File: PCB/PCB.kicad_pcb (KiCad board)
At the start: 6 copper layers, 22 x 80 mm, 269 parts, among them J1 Bus_M.2_Edge_M, J2 Conn_ARM_SWD_TagConnect_TC2030, J4 TYPE-C-31-M-12, J7 HDMI_D_1.4, SW1 SW_Push, U1 XC7A50T-FGG484, U10 FT2232HQ, U11 MT41J128M16JT-125:K, U12 PCA9306DC1, U14 UCL0524P, U15 UCL0524P, U16 UCL0524P, U17 TPS62132, U2 MAX20029ATIA/V+, U3 TPD2EUSB30, U4 TPD2EUSB30, U5 TPS2121RUXR, U6 TPD2EUSB30, U7 MT25QL128ABA1EW7-0SIT, U9 M93C56-WMN6TP, Y2 12MHz, Y3 100MHz

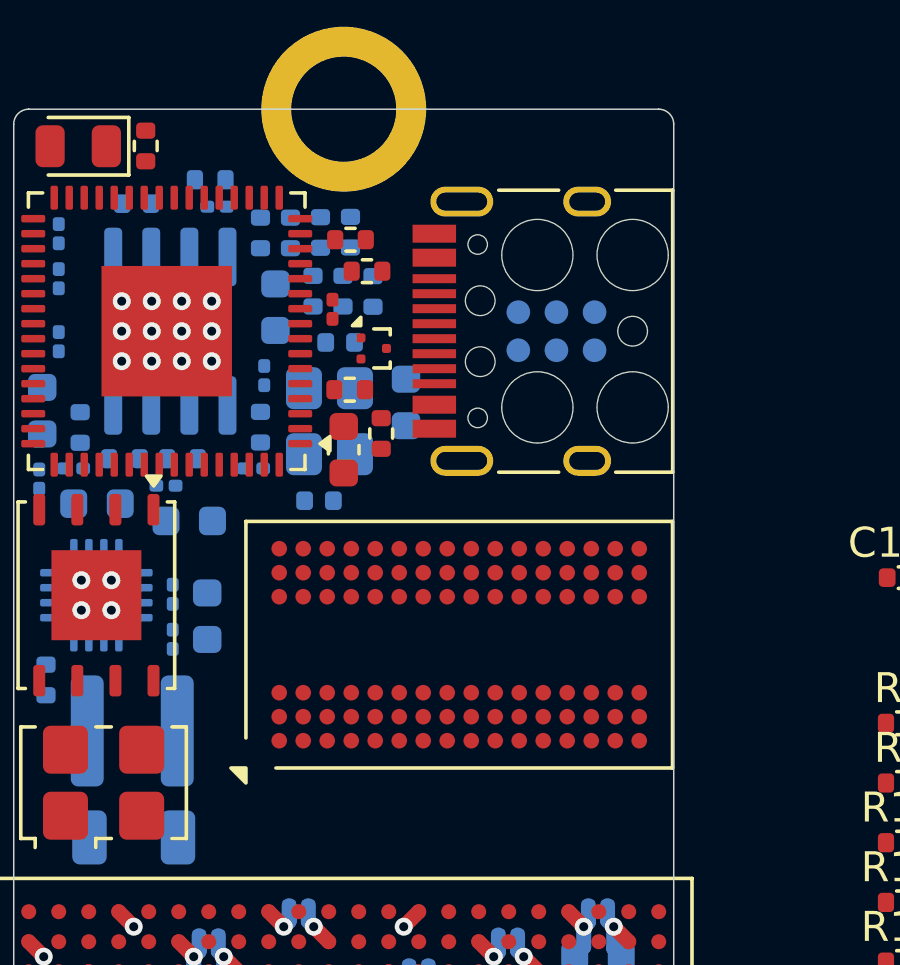
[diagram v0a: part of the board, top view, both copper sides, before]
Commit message: getting ready for DDR routing
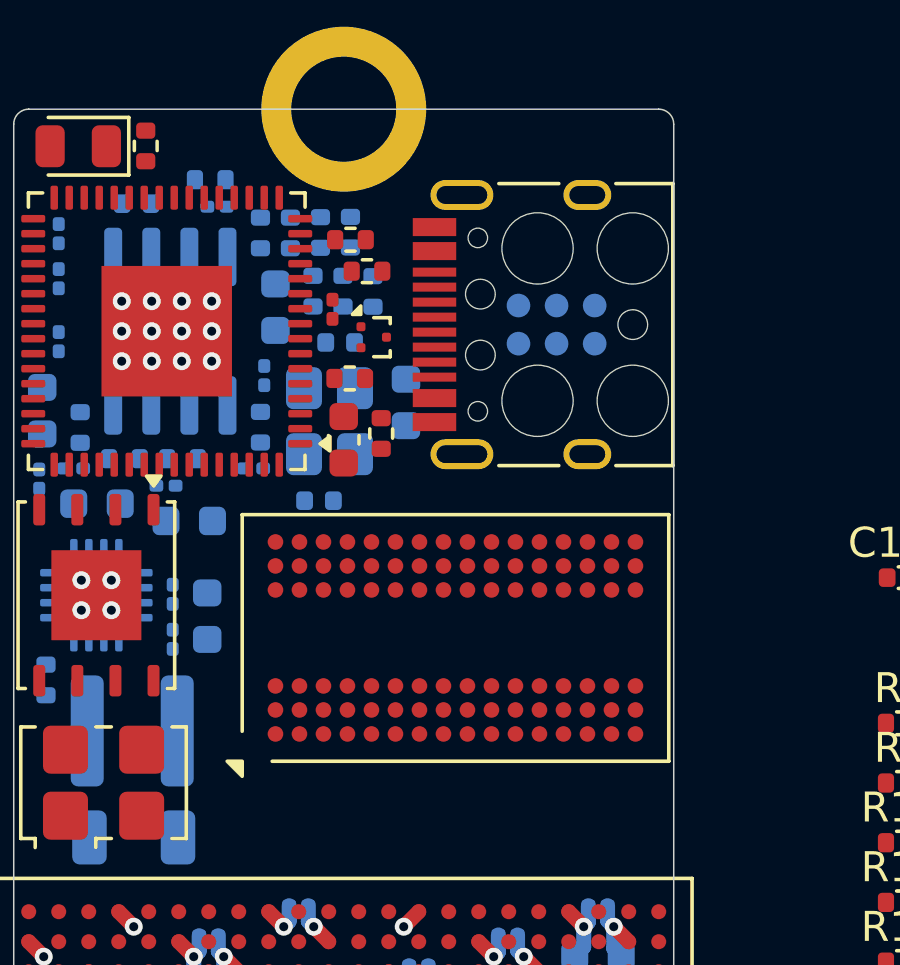
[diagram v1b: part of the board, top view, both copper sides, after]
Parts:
- moved R55 0.38 mm to (143.9, 69.2)
- moved U3 0.38 mm to (144.8, 67.8)
- moved C101 0.33 mm to (143.8, 71.3)
- moved U11 0.26 mm to (147.5, 77.9)
- moved J2 0.22 mm to (150.8, 67.4)
- moved J4 0.22 mm to (150.8, 67.4)
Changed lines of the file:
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@@
 	(footprint "Package_TO_SOT_SMD:Texas_DRT-3"
 		(layer "F.Cu")
-		(at 144.75 68.225 -90)
+		(at 144.75 67.85 -90)
 		(descr "Texas Instrument DRT-3 1x0.8mm Pitch 0.7mm http://www.ti.com/lit/ds/symlink/tpd2eusb30.pdf")
 		(tags "DRT-3 1x0.8mm Pitch 0.7mm")
@@
 	(footprint "Resistor_SMD:R_0402_1005Metric"
 		(layer "F.Cu")
-		(at 143.95 69.6 180)
+		(at 143.95 69.225 180)
 		(descr "Resistor SMD 0402 (1005 Metric), square (rectangular) end terminal, IPC-7351 nominal, (Body size source: IPC-SM-782 page 72, https://www.pcb-3d.com/wordpress/wp-content/uploads/ipc-sm-782a_amendment_1_and_2.pdf), generated with kicad-footprint-generator")
 		(tags "resistor")
@@
 	(footprint "Capacitor_SMD:C_0603_1608Metric"
 		(layer "F.Cu")
-		(at 143.75 71.6 -90)
+		(at 143.75 71.27 -90)
 		(descr "Capacitor SMD 0603 (1608 Metric), square (rectangular) end terminal, IPC-7351 nominal, (Body size source: IPC-SM-782 page 76, https://www.pcb-3d.com/wordpress/wp-content/uploads/ipc-sm-782a_amendment_1_and_2.pdf), generated with kicad-footprint-generator")
 		(tags "capacitor")
@@
 	(footprint "Package_BGA:Micron_FBGA-96_8x14mm_Layout9x16_P0.8mm"
 		(layer "F.Cu")
-		(at 147.6 78.1 90)
+		(at 147.475 77.875 90)
 		(descr "FBGA-96, 8.0x14.0mm, 96 Ball, 9x16 Layout, 0.8mm Pitch, generated with kicad-footprint-generator ipc_bga_generator.py, https://www.micron.com/-/media/client/global/documents/products/data-sheet/dram/ddr3/4gb_ddr3l.pdf#page=28")
 		(tags "BGA 96 0.8 DDR3 DDR3L DDR4")
@@
 	(footprint "Connector_USB:USB_C_Receptacle_HRO_TYPE-C-31-M-12"
 		(layer "F.Cu")
-		(at 150.815 67.65 90)
+		(at 150.82 67.43 90)
 		(descr "USB Type-C receptacle for USB 2.0 and PD, http://www.krhro.com/uploads/soft/180320/1-1P320120243.pdf")
 		(tags "usb usb-c 2.0 pd")
@@
 	(footprint "Connector:Tag-Connect_TC2030-IDC-FP_2x03_P1.27mm_Vertical"
 		(layer "B.Cu")
-		(at 150.84 67.65 180)
+		(at 150.845 67.43 180)
 		(descr "Tag-Connect programming header; http://www.tag-connect.com/Materials/TC2030-IDC.pdf")
 		(tags "tag connect programming header pogo pins")
@@
 			(polygon
 				(pts
-					(xy 149.57 67.015) (xy 152.11 67.015) (xy 152.11 68.285) (xy 149.57 68.285)
+					(xy 149.575 66.795) (xy 152.115 66.795) (xy 152.115 68.065) (xy 149.575 68.065)
 				)
 			)
